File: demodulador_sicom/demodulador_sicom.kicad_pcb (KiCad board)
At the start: 2 copper layers, 50 x 50 mm, 33 parts, among them J1 POWER, J2 OUTPUT, J3 CARRIER_IN, J4 SSB_IN, U1 MC1496D, U2 L7812

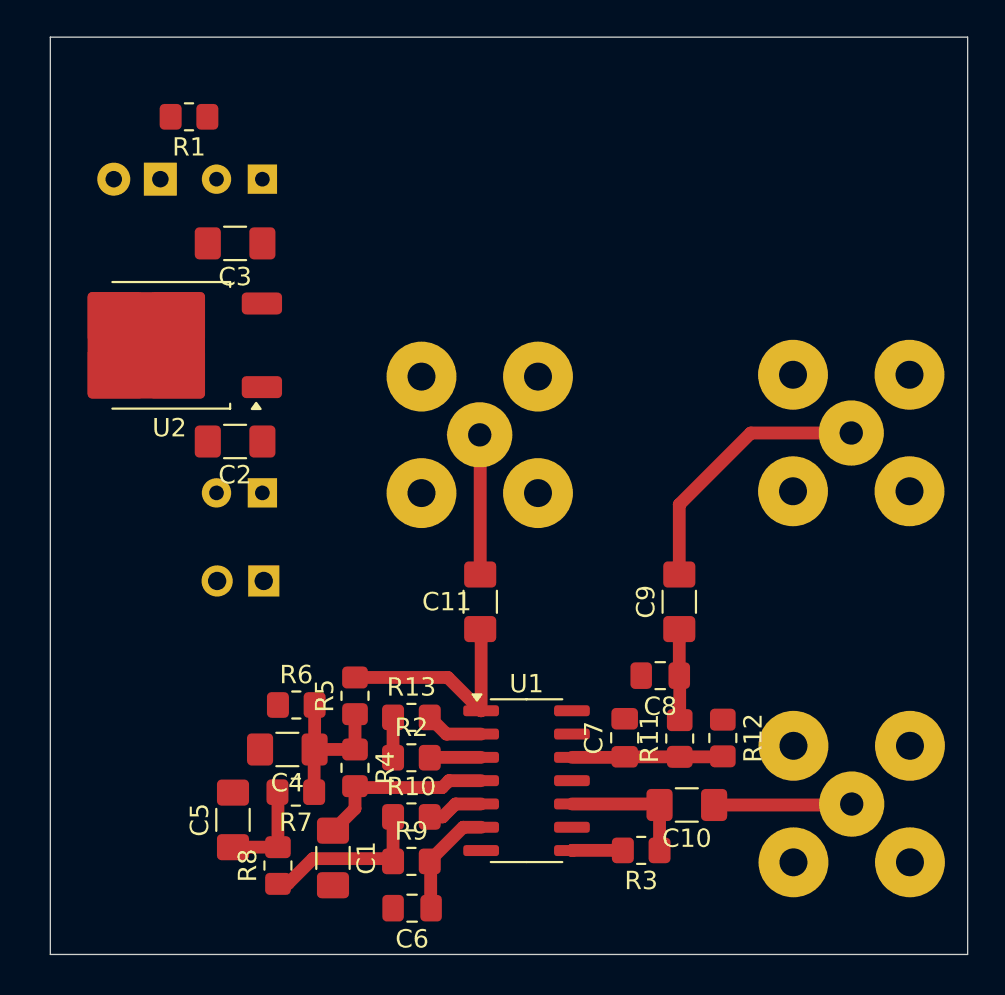
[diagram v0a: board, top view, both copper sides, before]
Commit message: Update pcb layout.
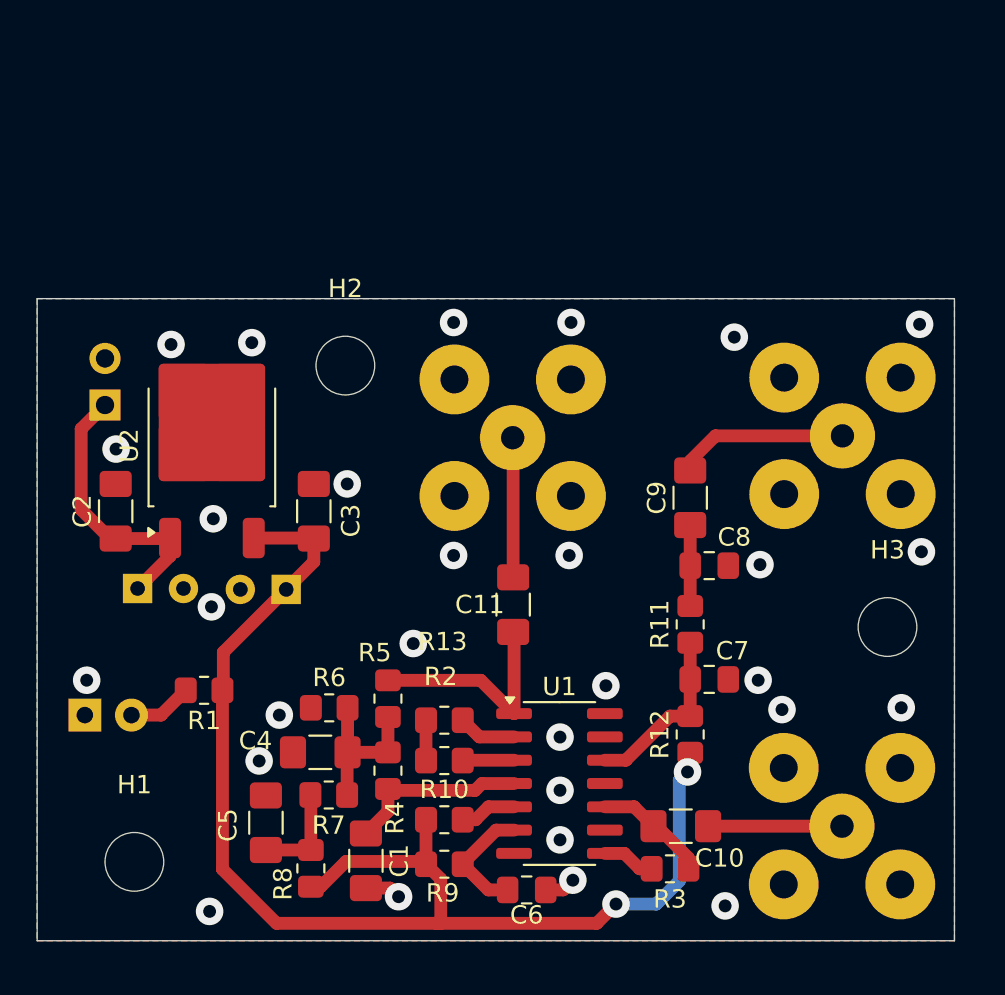
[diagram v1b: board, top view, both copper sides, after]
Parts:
- added H1: MountingHole, MountingHole:MountingHole_3.2mm_M3, F.Cu at (142.3, 119.4)
- added H2: MountingHole, MountingHole:MountingHole_3.2mm_M3, F.Cu at (153.8, 92.3)
- added H3: MountingHole, MountingHole:MountingHole_3.2mm_M3, F.Cu at (183.3, 106.6)
- moved R1 31.3 mm to (146.1, 110.0)
- moved D1 29.5 mm to (139.6, 111.4), turned to 0 degrees
- moved C12 22.4 mm to (150.6, 104.5)
- moved C3 15.2 mm to (152.1, 100.3), turned to 90 degrees
- moved J1 12.9 mm to (140.7, 94.5), turned to 0 degrees
- moved C13 8.57 mm to (142.5, 104.5), turned to 0 degrees
- moved C2 7.54 mm to (141.3, 100.3), turned to 90 degrees
- moved C8 6.56 mm to (173.6, 103.3), turned to 0 degrees
- moved C6 6.32 mm to (163.7, 120.9), turned to 0 degrees
- moved R11 6.25 mm to (172.6, 106.5)
- moved U2 5.94 mm to (146.5, 96.7), turned to 90 degrees
- moved C9 5.70 mm to (172.6, 99.6)
- moved C7 5.60 mm to (173.6, 109.5), turned to 0 degrees
- moved R3 1.86 mm to (171.5, 119.8)
- moved C4 1.80 mm to (152.4, 113.4)
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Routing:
- net +12V: track 9.33 -> 70.8 mm, vias 0 -> 2
- net /V_IN: track 0.00 -> 15.2 mm
- net /OUTPUT: track 14.8 -> 9.38 mm
- net GND: track 0.00 -> 3.67 mm, vias 0 -> 29
- net Net-(D1-A): track 0.00 -> 3.52 mm
- net /OUPUT_B: track 8.25 -> 9.65 mm
- net /CARRIER_A: track 7.27 -> 6.30 mm
- net Net-(C6-Pad1): track 5.83 -> 6.55 mm
- net /OUTPUT_A: track 4.97 -> 4.41 mm
- added copper zone on B.Cu, net GND
- added copper zone on F.Cu, net GND
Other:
- board size 50 x 50 mm -> 50 x 35 mm
